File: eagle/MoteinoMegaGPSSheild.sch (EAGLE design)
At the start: 32 parts, among them J1 BilgeSwitch, J2 Button, J3 LED, J4 DS18B20, J5 DS18B20, J6 GND, J7 OKI-78SR-5/1.5, J8 5V, J9 12-24V_VCC, Q1 NDP6020P, Q2 IRF9Z14PBF, Q3 2N7000, Q4 IRF9Z14PBF, Q5 2N7000

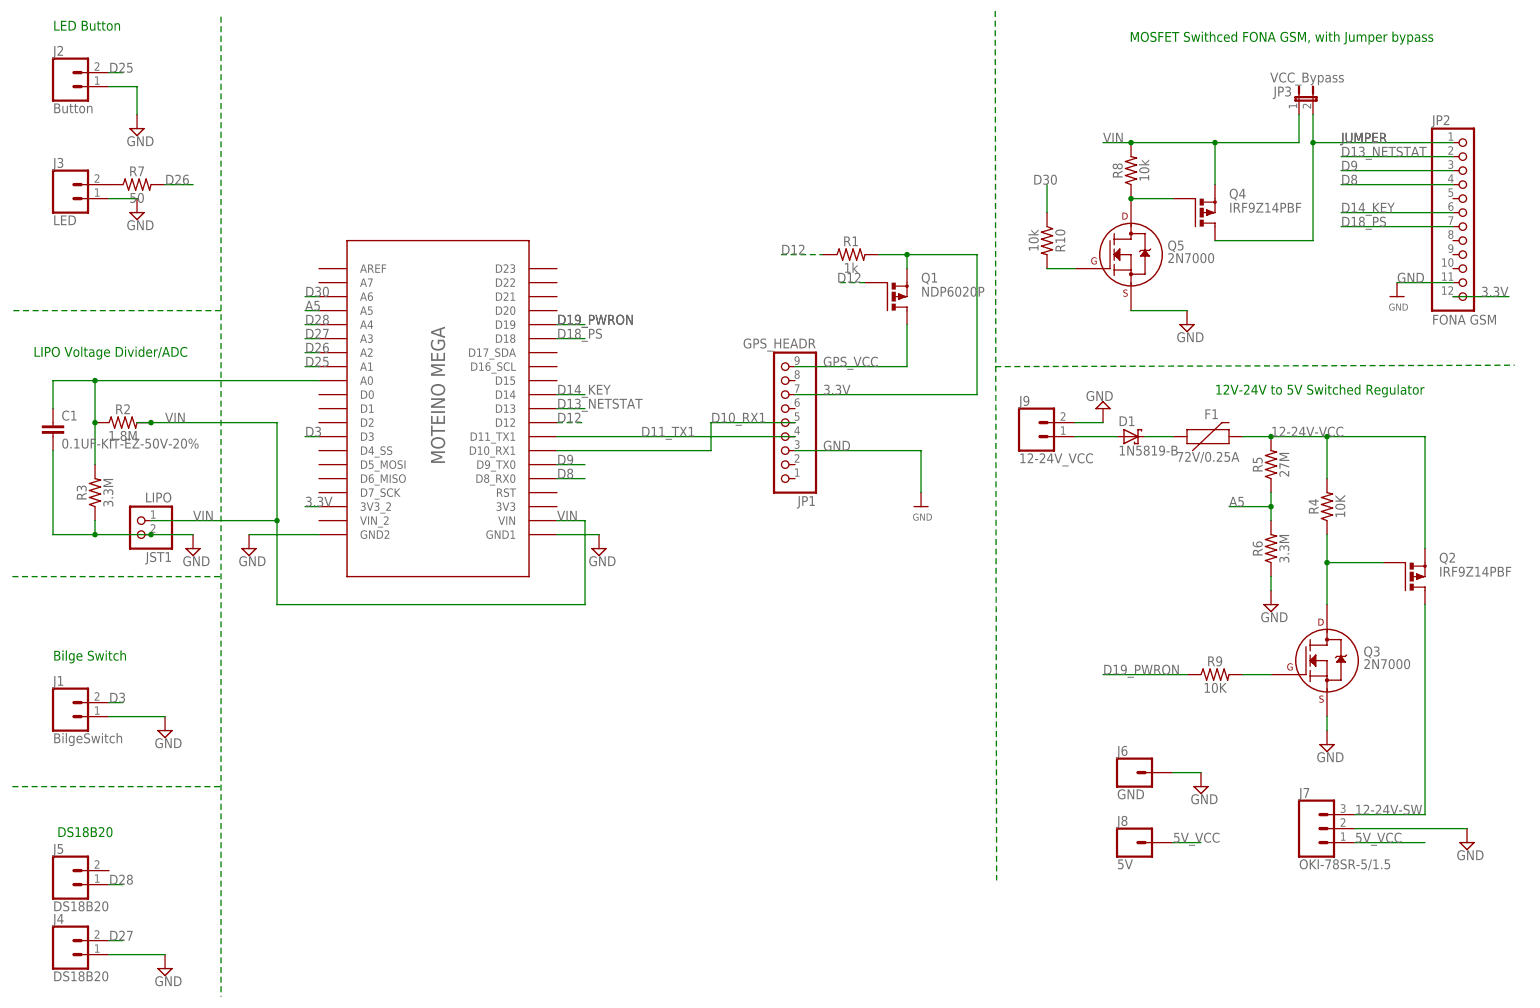
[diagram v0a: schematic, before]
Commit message: eagle updates
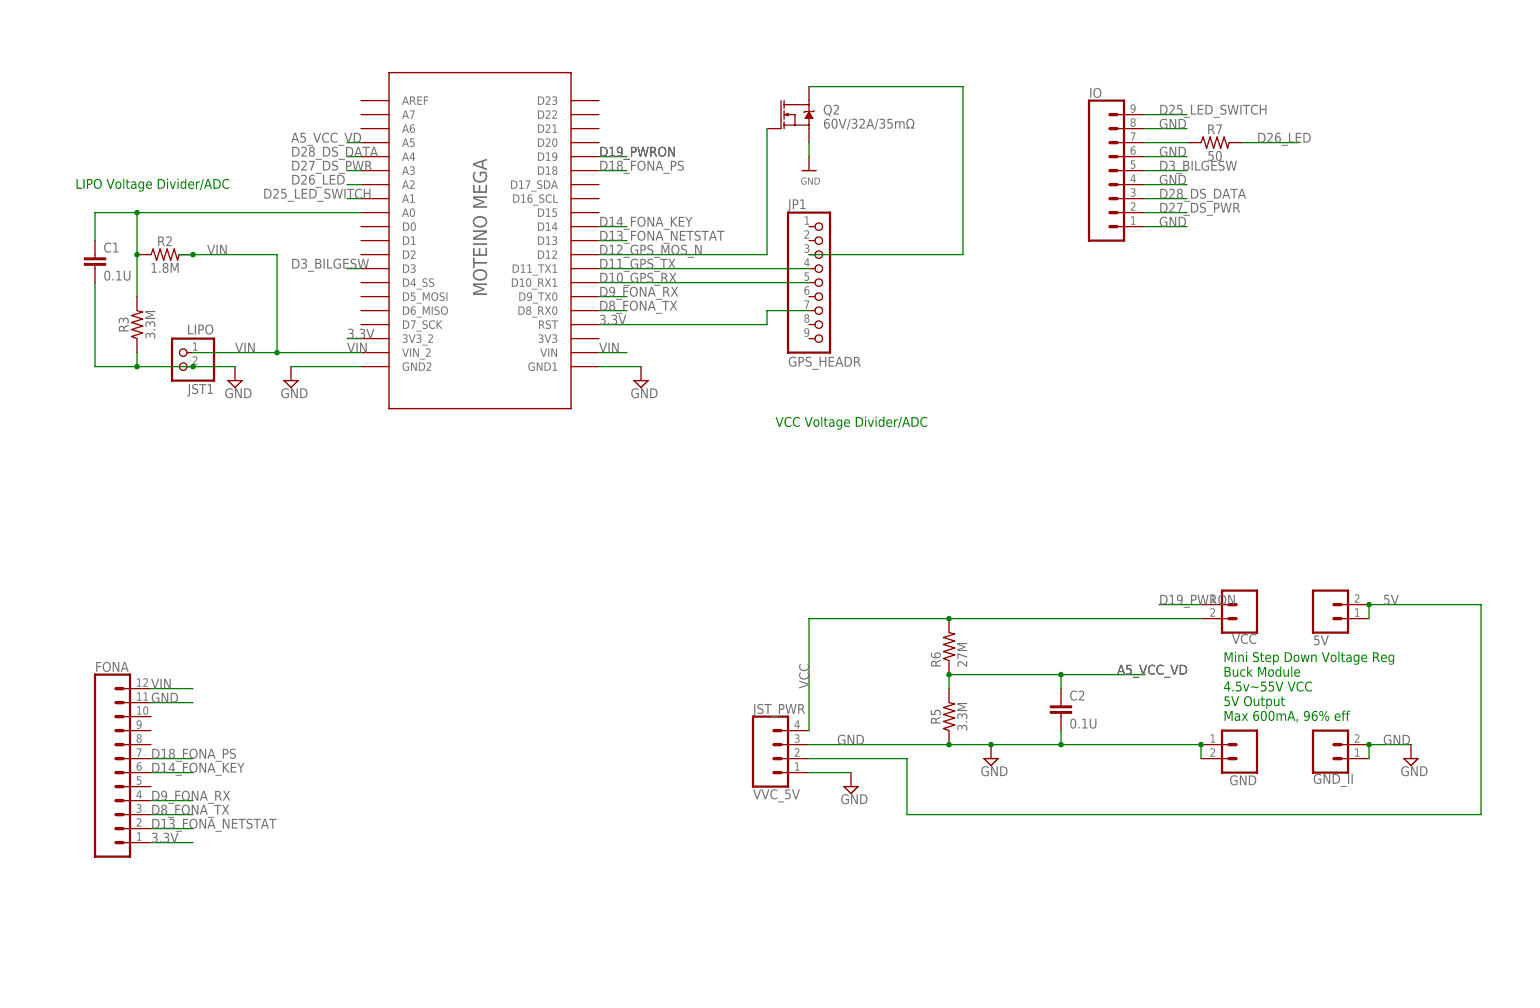
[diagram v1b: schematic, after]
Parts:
- removed D1: 1N5819-B, diode:1N5819-B
- removed F1: 72V/0.25A, SparkFun-Fuses:PPTC_PTH
- removed J1: BilgeSwitch, SparkFun-Connectors:CONN_023.5MM-NO_SILK
- removed J2: Button, SparkFun-Connectors:CONN_023.5MM-NO_SILK
- removed J3: LED, SparkFun-Connectors:CONN_023.5MM-NO_SILK
- removed J4, J5: DS18B20, SparkFun-Connectors:CONN_023.5MM-NO_SILK
- removed J6: GND, SparkFun-Connectors:CONN_01
- removed J7: OKI-78SR-5/1.5, SparkFun-Connectors:CONN_03
- removed J8: 5V, SparkFun-Connectors:CONN_01
- removed J9: 12-24V_VCC, SparkFun-Connectors:CONN_023.5MM-NO_SILK
- removed JP2: FONA GSM, adafruit2:PINHD-1X12-CB
- removed JP3: VCC_Bypass, jumper:JP1E
- removed Q1: NDP6020P, transistor-power:PMOSFET_PTO220BV
- removed Q3, Q5: 2N7000, transistors:2N7002_TO92
- removed Q4: IRF9Z14PBF, transistor-power:PMOSFET_PTO220BV
- removed R1: 1k, SparkFun-Resistors:1KOHM-HORIZ-1/4W-1%
- removed R10, R8: 10k, SparkFun-Resistors:1KOHM-HORIZ-1/4W-1%
- removed R4, R9: 10K, SparkFun-Resistors:1KOHM-HORIZ-1/4W-1%
- added 5V: 5V, SparkFun-Connectors:CONN_02
- added C2: 0.1U, SparkFun-Capacitors:0.1UF-KIT-EZ-50V-20%
- added FONA: (no value), SparkFun-Connectors:CONN_12
- added GND, GND_II: GND, SparkFun-Connectors:CONN_02
- added IO: (no value), SparkFun-Connectors:CONN_09
- added JST_PWR: VVC_5V, SparkFun-Connectors:CONN_04JST-PTH
- added VCC: VCC, SparkFun-Connectors:CONN_02
- C1: value 0.1UF-KIT-EZ-50V-20% -> 0.1U
- Q2: value IRF9Z14PBF -> 60V/32A/35mΩ; device transistor-power:PMOSFET_PTO220BV -> SparkFun-DiscreteSemi:MOSFET-NCH-FQP30N06L
- R5: value 27M -> 3.3M
- R6: value 3.3M -> 27M; device SparkFun-Resistors:1KOHM-HORIZ-1/4W-1% -> adafruit:R-US_0309/12
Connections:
- net D10_RX1 renamed D10_GPS_RX
- net D11_TX1 renamed D11_GPS_TX
- net D26 renamed D26_LED
- removed net 12-24V-SW: J7.3, Q2.D
- removed net 12-24V-VCC: F1.2, Q2.S, R4.2, R5.2
- removed net 5V_VCC: J7.1, J8.1
- removed net A5: MOTEINO_MEGA.A5, R5.1, R6.2
- removed net D12: MOTEINO_MEGA.D12, Q1.G, R1.1
- removed net D13_NETSTAT: JP2.2, MOTEINO_MEGA.D13
- removed net D14_KEY: JP2.6, MOTEINO_MEGA.D14
- removed net D18_PS: JP2.7, MOTEINO_MEGA.D18
- removed net D25: J2.2, MOTEINO_MEGA.A1
- removed net D27: J4.2, MOTEINO_MEGA.A3
- removed net D28: J5.1, MOTEINO_MEGA.A4
- removed net D3: J1.2, MOTEINO_MEGA.D3
- removed net D30: MOTEINO_MEGA.A6, R10.1
- removed net D8: JP2.4, MOTEINO_MEGA.D8_RX0
- removed net D9: JP2.3, MOTEINO_MEGA.D9_TX0
- removed net GPS_VCC: JP1.9, Q1.D
- removed net JUMPER: JP2.1, JP3.2, Q4.D
- removed net N$10: Q5.G, R10.2
- removed net N$5: Q4.G, Q5.D, R8.1
- removed net N$6: D1.A, J9.1
- removed net N$7: J3.2, R7.1
- removed net N$8: D1.C, F1.1
- removed net N$9: Q3.G, R9.2
- removed net SPEAKER2+: JP2.10
- new net 5V: 5V.1, 5V.2, JST_PWR.2
- new net A5_VCC_VD: C2.1, MOTEINO_MEGA.A5, R5.2, R6.1
- new net D12_GPS_MOS_N: MOTEINO_MEGA.D12, Q2.G
- new net D13_FONA_NETSTAT: FONA.2, MOTEINO_MEGA.D13
- new net D14_FONA_KEY: FONA.6, MOTEINO_MEGA.D14
- new net D18_FONA_PS: FONA.7, MOTEINO_MEGA.D18
- new net D25_LED_SWITCH: IO.9, MOTEINO_MEGA.A1
- new net D27_DS_PWR: IO.2, MOTEINO_MEGA.A3
- new net D28_DS_DATA: IO.3, MOTEINO_MEGA.A4
- new net D3_BILGESW: IO.5, MOTEINO_MEGA.D3
- new net D8_FONA_TX: FONA.3, MOTEINO_MEGA.D8_RX0
- new net D9_FONA_RX: FONA.4, MOTEINO_MEGA.D9_TX0
- new net N$1: JP1.3, Q2.D
- new net VCC: JST_PWR.4, R6.2, VCC.2
- net 3.3V: now also FONA.1, MOTEINO_MEGA.RST; no longer JP2.12, Q1.S, R1.2
- net D19_PWRON: now also VCC.1; no longer R9.1
- net GND: now also C2.2, FONA.11, GND.1, GND.2, GND_II.1, GND_II.2, IO.1, IO.4, IO.6, IO.8, JST_PWR.1, JST_PWR.3, Q2.S, R5.1; no longer J1.1, J2.1, J3.1, J4.1, J6.1, J7.2, J9.2, JP1.3, JP2.11, Q3.S, Q5.S, R6.1
- net N$2: now also IO.7, R7.1; no longer Q2.G, Q3.D, R4.1
- net VIN: now also FONA.12, MOTEINO_MEGA.VIN_2; no longer JP3.1, Q4.S, R8.2
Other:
- note added: "Mini Step Down Voltage Reg Buck Module 4.5v~55V VCC 5V Output Max 600mA, 96% eff"
- note added: "VCC Voltage Divider/ADC"
- note removed: "12V-24V to 5V Switched Regulator"
- note removed: "Bilge Switch"
- note removed: "DS18B20"
- note removed: "LED Button"
- note removed: "MOSFET Swithced FONA GSM, with Jumper bypass"
- moved on the sheet: C1, JP1, JST1, R2, R3, R5, R6, R7
